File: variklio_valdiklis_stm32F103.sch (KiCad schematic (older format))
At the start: 88 parts, among them Q1 BC807, Q2 IRF830, Q3 IRF830, Q4 IRF830, Q5 IRF830, Q6 IRF830, Q7 IRF830, U1 CNY17-1, U10 IR2101, U2 CNY17-1, U3 CNY17-1, U4 LNK304G, U5 PC817, U6 SIP21106, U7 STM32F103C8Tx, U8 IR2101, U9 IR2101

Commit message: stm32f103c8tx schemos ir plokstes ruosimas
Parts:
- removed L2: 1mH/280mA, symbol Device:L
- added C1, C3, C4: 120x400V, Capacitor_THT:CP_Radial_D22.0mm_P10.00mm_SnapIn, symbol variklio_valdiklis_stm32F103-rescue:CP-Device
- added C14: 100n, Capacitor_SMD:C_0805_2012Metric, symbol variklio_valdiklis_stm32F103-rescue:C-Device
- added C24: 1n0, Capacitor_SMD:C_0805_2012Metric, symbol variklio_valdiklis_stm32F103-rescue:C-Device
- added D10, D20, D8, D9: LL4148, Diode_SMD:D_MiniMELF, symbol variklio_valdiklis_stm32F103-rescue:D-Device
- added D22, D23, D24, D25: D, Diode_THT:D_DO-201AD_P15.24mm_Horizontal, symbol variklio_valdiklis_stm32F103-rescue:D-Device
- added F1: 3A, Fuse:Fuseholder_TR5_Littelfuse_No560_No460, symbol Device:Fuse
- added F2: 5A, Fuse:Fuseholder_TR5_Littelfuse_No560_No460, symbol Device:Fuse
- added J1: Conn_01x05, valdiklio_footprints:Jungtis, symbol Connector_Generic:Conn_01x05
- added J3: ISP_SWD_Connector, mech:ISP_SWD_Connector, symbol mech:ISP_SWD_Connector
- added L2: 1mH/280mA, Inductor_THT:L_Radial_D7.8mm_P5.00mm_Fastron_07HCP, symbol Device:L_Core_Iron
- added R16: 100k, Resistor_SMD:R_0805_2012Metric, symbol variklio_valdiklis_stm32F103-rescue:R-Device
- added R18, R38, R39: 1K0, Resistor_SMD:R_0805_2012Metric, symbol variklio_valdiklis_stm32F103-rescue:R-Device
- added R19, R20, R21: 1k0, Resistor_SMD:R_0805_2012Metric, symbol variklio_valdiklis_stm32F103-rescue:R-Device
- added R34: 0R1, Resistor_THT:R_Axial_DIN0309_L9.0mm_D3.2mm_P12.70mm_Horizontal, symbol variklio_valdiklis_stm32F103-rescue:R_US-Device
- added R40: 220k, Resistor_THT:R_Axial_DIN0411_L9.9mm_D3.6mm_P12.70mm_Horizontal, symbol variklio_valdiklis_stm32F103-rescue:R-Device
- added RV1, RV2: Varistor, Varistor:RV_Disc_D9mm_W4mm_P5mm, symbol Device:Varistor
- added TH1: 33R, Varistor:RV_Disc_D9mm_W4mm_P5mm, symbol Device:Thermistor_PTC
- added TH2: 10K, symbol Device:Thermistor_NTC
- C10: renamed from C?; symbol Device:C -> variklio_valdiklis_stm32F103-rescue:C-Device
- C11: renamed from C7; symbol Device:C -> variklio_valdiklis_stm32F103-rescue:C-Device
- C12: renamed from C8; value 0.1 -> 100n; symbol Device:C -> variklio_valdiklis_stm32F103-rescue:C-Device
- C13: renamed from C9; footprint Capacitor_THT:C_Radial_D6.3mm_H5.0mm_P2.50mm -> Capacitor_THT:CP_Radial_D6.3mm_P2.50mm; symbol Device:CP -> variklio_valdiklis_stm32F103-rescue:CP-Device
- C15: renamed from C10; value C -> 100n; symbol Device:C -> variklio_valdiklis_stm32F103-rescue:C-Device
- C16: renamed from C11; value C -> 100n; symbol Device:C -> variklio_valdiklis_stm32F103-rescue:C-Device
- C17: renamed from C12; value C -> 100n; symbol Device:C -> variklio_valdiklis_stm32F103-rescue:C-Device
- C18: renamed from C13; symbol Device:C -> variklio_valdiklis_stm32F103-rescue:C-Device
- C19: renamed from C14; symbol Device:C -> variklio_valdiklis_stm32F103-rescue:C-Device
- C2: renamed from C1; footprint Capacitor_THT:C_Radial_D10.0mm_H20.0mm_P5.00mm -> Capacitor_THT:CP_Radial_D10.0mm_P5.00mm; symbol Device:CP -> variklio_valdiklis_stm32F103-rescue:CP-Device
- C20: renamed from C15; symbol Device:C -> variklio_valdiklis_stm32F103-rescue:C-Device
- C21: renamed from C16; symbol Device:C -> variklio_valdiklis_stm32F103-rescue:C-Device
- C22: renamed from C17; symbol Device:C -> variklio_valdiklis_stm32F103-rescue:C-Device
- C23: renamed from C18; symbol Device:C -> variklio_valdiklis_stm32F103-rescue:C-Device
- C5: renamed from C2; footprint Capacitor_THT:C_Radial_D10.0mm_H20.0mm_P5.00mm -> Capacitor_THT:CP_Radial_D10.0mm_P5.00mm; symbol Device:CP -> variklio_valdiklis_stm32F103-rescue:CP-Device
- C6: renamed from C5; symbol Device:CP -> variklio_valdiklis_stm32F103-rescue:CP-Device
- C7: renamed from C3; symbol Device:C -> variklio_valdiklis_stm32F103-rescue:C-Device
- C8: renamed from C4; footprint Capacitor_THT:C_Radial_D6.3mm_H5.0mm_P2.50mm -> Capacitor_THT:CP_Radial_D6.3mm_P2.50mm; symbol Device:CP -> variklio_valdiklis_stm32F103-rescue:CP-Device
- C9: renamed from C6; symbol Device:C -> variklio_valdiklis_stm32F103-rescue:C-Device
- D11: renamed from D6; value US1J -> UF4005; footprint (none) -> Diode_THT:D_DO-41_SOD81_P7.62mm_Horizontal; symbol Device:D -> variklio_valdiklis_stm32F103-rescue:D-Device
- D12: renamed from D7; value US1J -> UF4005; footprint (none) -> Diode_THT:D_DO-41_SOD81_P7.62mm_Horizontal; symbol Device:D -> variklio_valdiklis_stm32F103-rescue:D-Device
- D13: renamed from D8; value US1J -> UF4005; footprint (none) -> Diode_THT:D_DO-41_SOD81_P7.62mm_Horizontal; symbol Device:D -> variklio_valdiklis_stm32F103-rescue:D-Device
- D14: renamed from D9; footprint (none) -> Diode_SMD:D_MiniMELF; symbol Device:D -> variklio_valdiklis_stm32F103-rescue:D-Device
- D15: renamed from D10; footprint (none) -> Diode_SMD:D_MiniMELF; symbol Device:D -> variklio_valdiklis_stm32F103-rescue:D-Device
- D16: renamed from D11; footprint (none) -> Diode_SMD:D_MiniMELF; symbol Device:D -> variklio_valdiklis_stm32F103-rescue:D-Device
- D17: renamed from D12; footprint (none) -> Diode_SMD:D_MiniMELF; symbol Device:D -> variklio_valdiklis_stm32F103-rescue:D-Device
- D18: renamed from D13; footprint (none) -> Diode_SMD:D_MiniMELF; symbol Device:D -> variklio_valdiklis_stm32F103-rescue:D-Device
- D19: renamed from D14; footprint (none) -> Diode_SMD:D_MiniMELF; symbol Device:D -> variklio_valdiklis_stm32F103-rescue:D-Device
- D2: renamed from D1; symbol Device:D -> variklio_valdiklis_stm32F103-rescue:D-Device
- D3: renamed from D2; symbol Device:D -> variklio_valdiklis_stm32F103-rescue:D-Device
- D4: renamed from D3; value LL4005 -> LL4148; footprint Diode_SMD:D_MELF -> Diode_SMD:D_MiniMELF; symbol Device:D -> variklio_valdiklis_stm32F103-rescue:D-Device
- D5: renamed from D4; footprint (none) -> Diode_THT:D_DO-41_SOD81_P10.16mm_Horizontal; symbol Device:D -> variklio_valdiklis_stm32F103-rescue:D-Device
- D6: renamed from D5; value D_Zener -> 12V; footprint (none) -> Diode_SMD:D_MiniMELF; symbol Device:D_Zener -> variklio_valdiklis_stm32F103-rescue:D_Zener-Device
- D7: renamed from D?; value LL4005 -> LL4148; footprint Diode_SMD:D_MELF -> Diode_SMD:D_MiniMELF; symbol Device:D -> variklio_valdiklis_stm32F103-rescue:D-Device
- L1: footprint (none) -> Inductor_SMD:L_Vishay_IHSM-3825; symbol Device:L -> variklio_valdiklis_stm32F103-rescue:L-Device
- Q1: symbol Transistor_BJT:BC807 -> variklio_valdiklis_stm32F103-rescue:BC807-Transistor_BJT
- Q2, Q3, Q4, Q5, Q6, Q7: symbol Transistor_FET:IRF740 -> variklio_valdiklis_stm32F103-rescue:IRF740-Transistor_FET
- R1: renamed from R2; symbol Device:R -> variklio_valdiklis_stm32F103-rescue:R-Device
- R10, R11, R12, R13, R14, R15, R5, R6: symbol Device:R -> variklio_valdiklis_stm32F103-rescue:R-Device
- R17: renamed from R?; symbol Device:R -> variklio_valdiklis_stm32F103-rescue:R-Device
- R2: renamed from R3; symbol Device:R -> variklio_valdiklis_stm32F103-rescue:R-Device
- R22: renamed from R16; value R -> 47R; symbol Device:R -> variklio_valdiklis_stm32F103-rescue:R-Device
- R23: renamed from R17; value R -> 47R; symbol Device:R -> variklio_valdiklis_stm32F103-rescue:R-Device
- R24: renamed from R18; value R -> 47R; symbol Device:R -> variklio_valdiklis_stm32F103-rescue:R-Device
- R25: renamed from R19; value R -> 47R; symbol Device:R -> variklio_valdiklis_stm32F103-rescue:R-Device
- R26: renamed from R20; value R -> 47R; symbol Device:R -> variklio_valdiklis_stm32F103-rescue:R-Device
- R27: renamed from R21; value R -> 47R; symbol Device:R -> variklio_valdiklis_stm32F103-rescue:R-Device
- R28: renamed from R22; symbol Device:R -> variklio_valdiklis_stm32F103-rescue:R-Device
- R29: renamed from R23; symbol Device:R -> variklio_valdiklis_stm32F103-rescue:R-Device
- R3: renamed from R4; symbol Device:R -> variklio_valdiklis_stm32F103-rescue:R-Device
- R30: renamed from R24; symbol Device:R -> variklio_valdiklis_stm32F103-rescue:R-Device
- R31: renamed from R25; symbol Device:R -> variklio_valdiklis_stm32F103-rescue:R-Device
- R32: renamed from R26; symbol Device:R -> variklio_valdiklis_stm32F103-rescue:R-Device
- R33: renamed from R27; symbol Device:R -> variklio_valdiklis_stm32F103-rescue:R-Device
- R35: renamed from R28; symbol Device:R_US -> variklio_valdiklis_stm32F103-rescue:R_US-Device
- R36: renamed from R29; symbol Device:R_US -> variklio_valdiklis_stm32F103-rescue:R_US-Device
- R37: renamed from R30; symbol Device:R_US -> variklio_valdiklis_stm32F103-rescue:R_US-Device
- R4: renamed from R1; footprint (none) -> Resistor_THT:R_Axial_DIN0411_L9.9mm_D3.6mm_P12.70mm_Horizontal; symbol Device:R -> variklio_valdiklis_stm32F103-rescue:R-Device
- R7: renamed from R8; symbol Device:R -> variklio_valdiklis_stm32F103-rescue:R-Device
- R8: renamed from R9; symbol Device:R -> variklio_valdiklis_stm32F103-rescue:R-Device
- R9: renamed from R7; symbol Device:R -> variklio_valdiklis_stm32F103-rescue:R-Device
- U1, U2, U3: symbol Isolator:CNY17-1 -> variklio_valdiklis_stm32F103-rescue:CNY17-1-Isolator
- U10, U8, U9: footprint (none) -> Package_SO:SOIC-8_3.9x4.9mm_P1.27mm; symbol Driver_FET:IR2101 -> variklio_valdiklis_stm32F103-rescue:IR2101-Driver_FET
- U4: symbol Regulator_Switching:LNK304G -> variklio_valdiklis_stm32F103-rescue:LNK304G-Regulator_Switching
- U5: footprint Package_DIP:DIP-4_W7.62mm -> Package_DIP:DIP-4_W10.16mm_LongPads; symbol Isolator:PC817 -> variklio_valdiklis_stm32F103-rescue:PC817-Isolator
- U6: footprint TO_SOT_Packages_SMD:SOT-23-5 -> Package_TO_SOT_SMD:SOT-23-5; symbol disc:USTAB_SIP21106-DT-33 -> variklio_valdiklis_stm32F103-rescue:USTAB_SIP21106-DT-33-disc
- VP1: symbol Device:R_POT_TRIM -> variklio_valdiklis_stm32F103-rescue:R_POT_TRIM-Device
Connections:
- net labels added: VB, ~NRST
- net labels removed: ~SA, ~SB, ~SC
- wire segments 350 -> 423
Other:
- moved on the sheet: C11, C12, C13, C15, C16, C17, C18, C19, C2, C20, C21, C22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

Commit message: 2019.10.10
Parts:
- J3: symbol mech:ISP_SWD_Connector -> variklio_valdiklis_stm32F103-rescue:ISP_SWD_Connector-mech
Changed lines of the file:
@@
 EESchema Schematic File Version 4
 LIBS:variklio_valdiklis_stm32F103-cache
-EELAYER 30 0
+EELAYER 29 0
 EELAYER END
 $Descr A3 16535 11693
@@
 	7950 3050 8500 3050
 $Comp
-L mech:ISP_SWD_Connector J3
+L variklio_valdiklis_stm32F103-rescue:ISP_SWD_Connector-mech J3
 U 1 1 5DDC24FE
 P 7950 2650

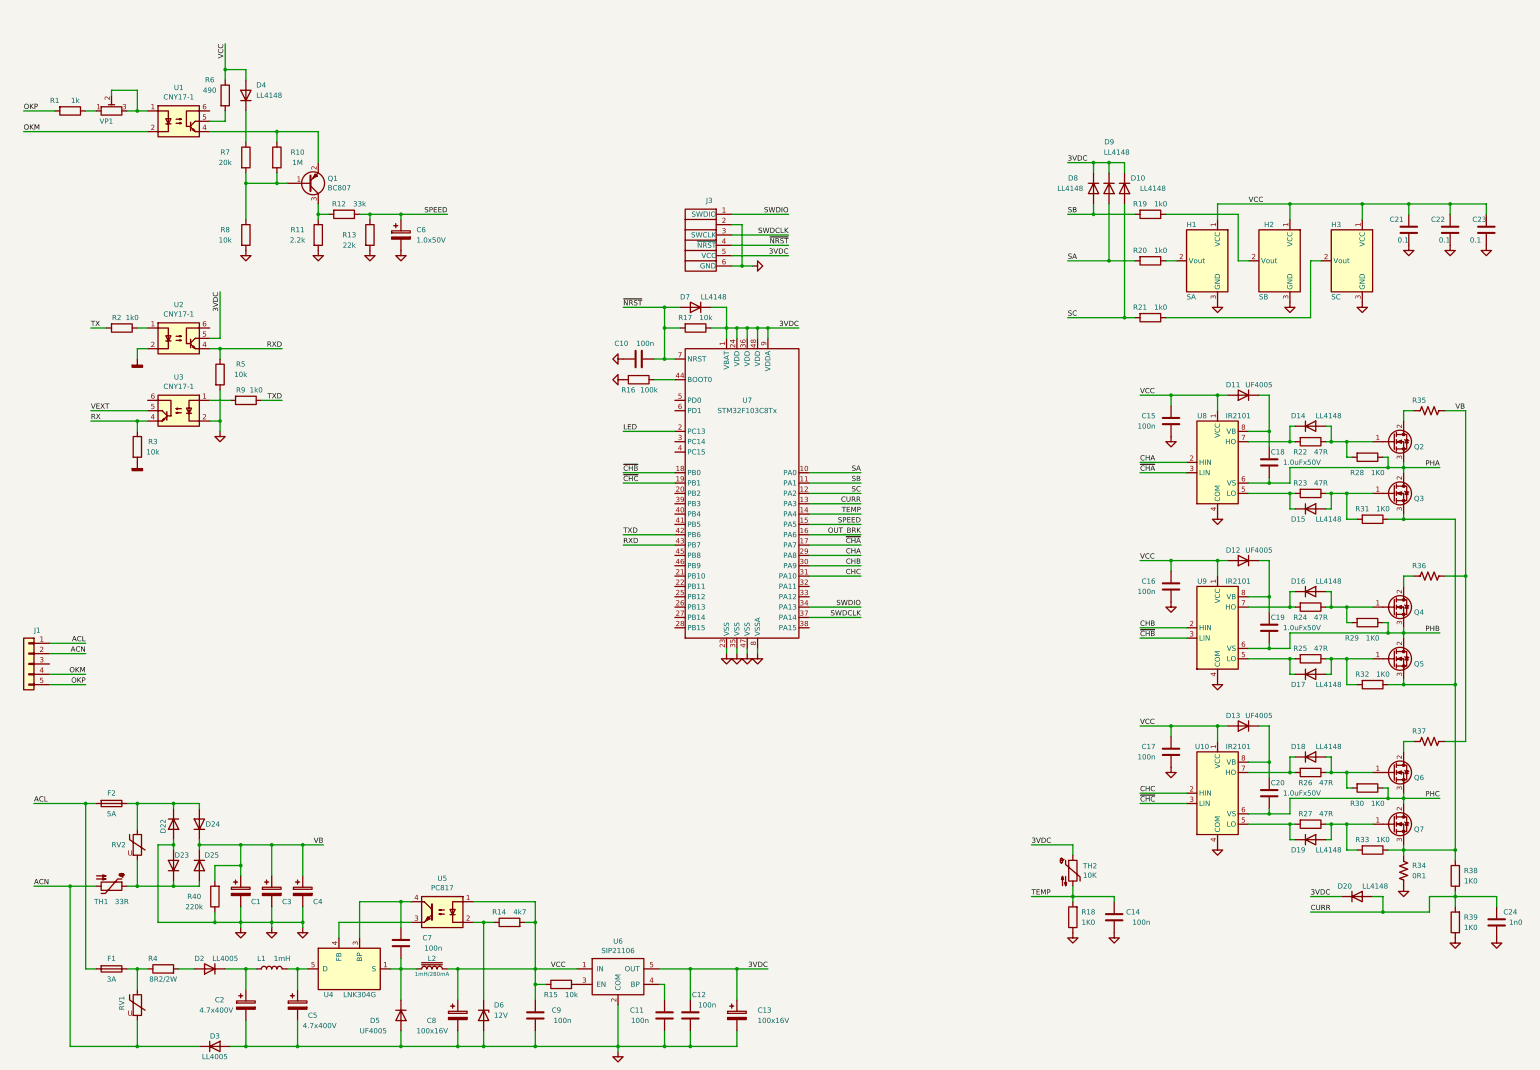
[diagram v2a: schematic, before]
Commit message: plokstes testavimams
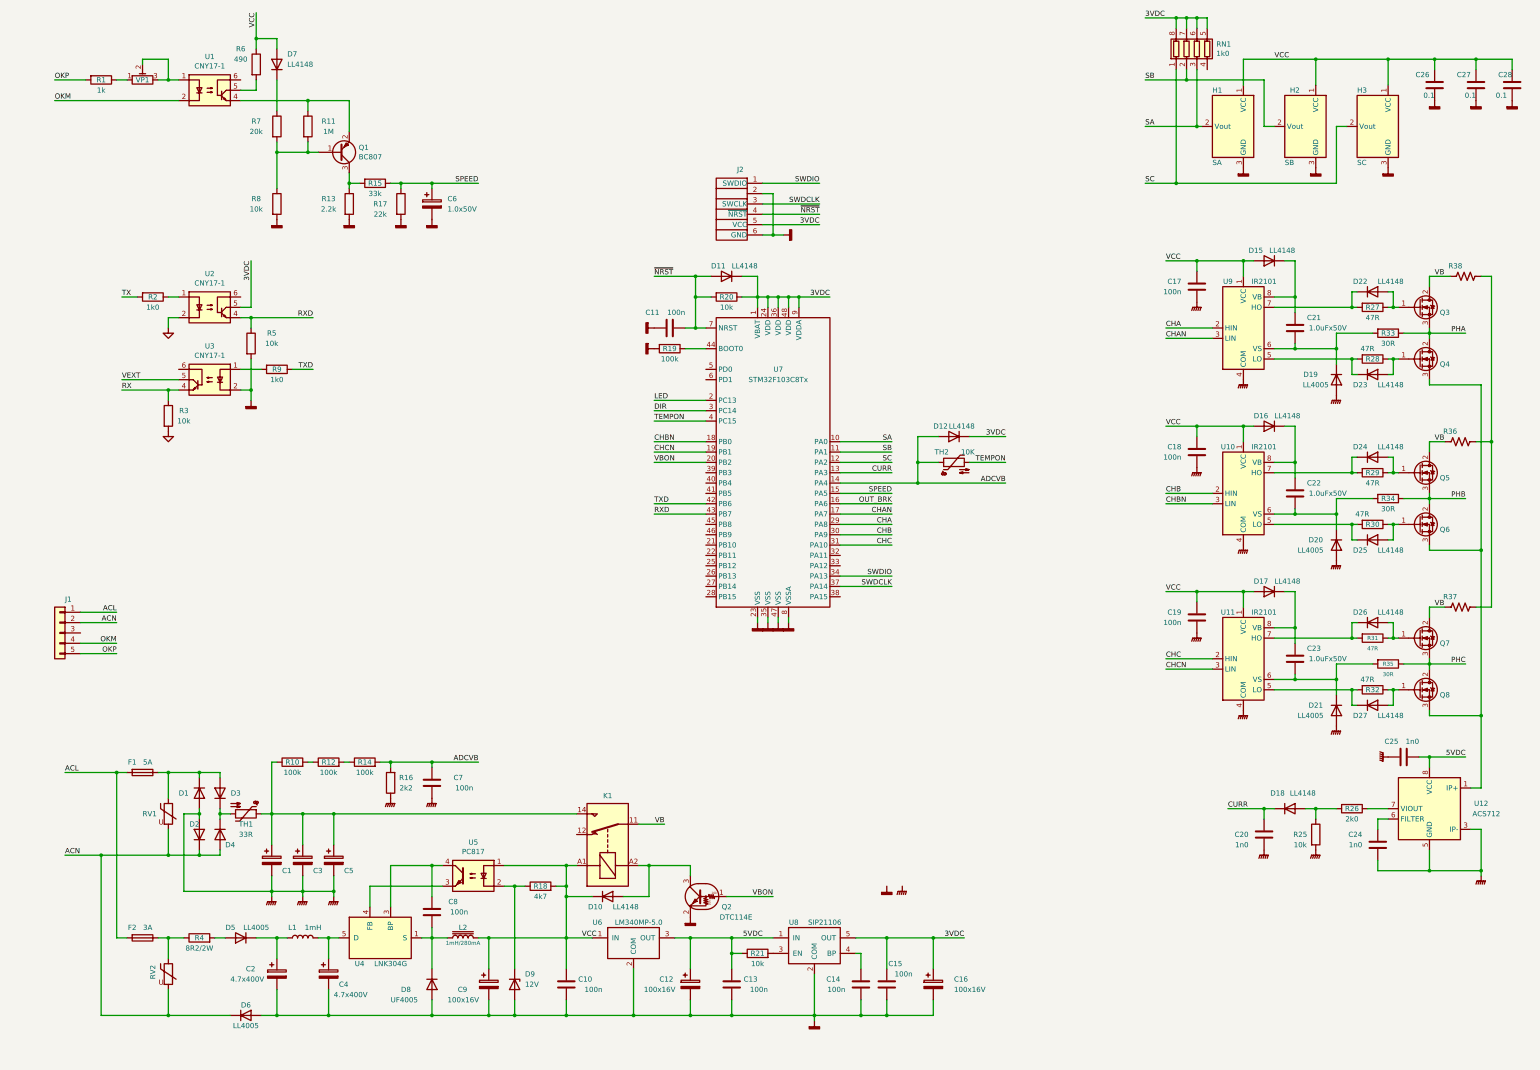
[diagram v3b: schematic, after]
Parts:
- removed C14: 100n, Capacitor_SMD:C_0805_2012Metric, symbol variklio_valdiklis_stm32F103-rescue:C-Device
- removed D20, D8, D9: LL4148, Diode_SMD:D_MiniMELF, symbol variklio_valdiklis_stm32F103-rescue:D-Device
- removed R18, R28, R29, R30, R31, R32, R39: 1K0, Resistor_SMD:R_0805_2012Metric, symbol variklio_valdiklis_stm32F103-rescue:R-Device
- removed R19, R20, R21: 1k0, Resistor_SMD:R_0805_2012Metric, symbol variklio_valdiklis_stm32F103-rescue:R-Device
- removed R34: 0R1, Resistor_THT:R_Axial_DIN0309_L9.0mm_D3.2mm_P12.70mm_Horizontal, symbol variklio_valdiklis_stm32F103-rescue:R_US-Device
- removed R40: 220k, Resistor_THT:R_Axial_DIN0411_L9.9mm_D3.6mm_P12.70mm_Horizontal, symbol variklio_valdiklis_stm32F103-rescue:R-Device
- added C12: 100x16V, Capacitor_THT:CP_Radial_D6.3mm_P2.50mm, symbol variklio_valdiklis_stm32F103-rescue:CP-Device
- added C13, C7: 100n, Capacitor_SMD:C_0805_2012Metric, symbol variklio_valdiklis_stm32F103-rescue:C-Device
- added C20, C25: 1n0, Capacitor_SMD:C_0805_2012Metric, symbol variklio_valdiklis_stm32F103-rescue:C-Device
- added D12, D15, D16, D17, D18: LL4148, Diode_SMD:D_MiniMELF, symbol variklio_valdiklis_stm32F103-rescue:D-Device
- added K1: Omron, Relay_THT:Relay_SPDT_Finder_34.51_Vertical, symbol Relay:FINDER-32.21-x000
- added Q2: DTC114E, Package_TO_SOT_SMD:SOT-23, symbol Transistor_BJT:DTC114E
- added R10, R12, R14: 100k, Resistor_SMD:R_1206_3216Metric, symbol variklio_valdiklis_stm32F103-rescue:R-Device
- added R16: 2k2, Resistor_SMD:R_0805_2012Metric, symbol variklio_valdiklis_stm32F103-rescue:R-Device
- added R25: 10k, Resistor_SMD:R_0805_2012Metric, symbol variklio_valdiklis_stm32F103-rescue:R-Device
- added R34, R35: 30R, Resistor_SMD:R_0805_2012Metric, symbol variklio_valdiklis_stm32F103-rescue:R-Device
- added RN1: 1k0, Resistor_SMD:R_Array_Convex_4x0603, symbol Device:R_Pack04
- added U12: ACS712, Package_SO:SOIC-8_3.9x4.9mm_P1.27mm, symbol Sensor_Current:ACS712xLCTR-05B
- added U6: LM340MP-5.0, disc:LM340_SOT-223, symbol disc:LM340MP-5.0
- D19: renamed from D11; value UF4005 -> LL4005; footprint Diode_THT:D_DO-41_SOD81_P7.62mm_Horizontal -> Diode_SMD:D_MELF
- D20: renamed from D12; value UF4005 -> LL4005; footprint Diode_THT:D_DO-41_SOD81_P7.62mm_Horizontal -> Diode_SMD:D_MELF
- D21: renamed from D13; value UF4005 -> LL4005; footprint Diode_THT:D_DO-41_SOD81_P7.62mm_Horizontal -> Diode_SMD:D_MELF
- R26: renamed from R38; value 1K0 -> 2k0
- R33: value 1K0 -> 30R
- renumbered C9 to C10, C10 to C11, C11 to C14, C12 to C15, C13 to C16, C15 to C17, C16 to C18, C17 to C19, C18 to C21, C19 to C22, C20 to C23, C21 to C26, C22 to C27, C23 to C28, C5 to C4, C4 to C5, C7 to C8, C8 to C9, D22 to D1, D7 to D11, D23 to D2, D14 to D22, D15 to D23, D16 to D24, D17 to D25, D18 to D26, D19 to D27, D24 to D3, D25 to D4, D2 to D5, D3 to D6, D4 to D7, D5 to D8, D6 to D9, F2 to F1, F1 to F2, J3 to J2, Q2 to Q3, Q3 to Q4, Q4 to Q5, Q5 to Q6, Q6 to Q7, Q7 to Q8, R10 to R11, R11 to R13, R12 to R15, R13 to R17, R14 to R18, R16 to R19, R17 to R20, R15 to R21, R22 to R27, R23 to R28, R24 to R29, R25 to R30, R26 to R31, R27 to R32, R35 to R38, RV2 to RV1, RV1 to RV2, U9 to U10, U10 to U11, U6 to U8, U8 to U9
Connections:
- net 3VDC: now also D12.1 (K), RN1.5 (R4.2), RN1.6 (R3.2), RN1.7 (R2.2), RN1.8 (R1.2); no longer D10.1 (K), TH2.1
- net ACN: now also D2.1 (K), D4.2 (A), RV1.2; no longer TH1.2
- net CURR: now also C20.2, D18.1 (K); no longer C24.2, R26.1
- net GND: now also R3.2, U2.2; no longer C1.2, C10.1, C11.1, C14.1, C15.1, C16.2, C17.1, C18.1, C19.1, C2.2, C24.1, C26.1, C27.1, C28.1, C3.2, C4.2, C5.2, C6.2, C9.2, D1.2 (A), D2.2 (A), D6.2 (A), D8.2 (A), D9.2 (A), H1.3 (GND), H2.3 (GND), H3.3 (GND), J2.2, J2.6 (GND), R13.2, R17.2, R19.2, R5.2, R8.2, U10.4 (COM), U11.4 (COM), U3.2, U7.23 (VSS), U7.35 (VSS), U7.47 (VSS), U7.8 (VSSA), U8.2 (COM), U9.4 (COM)
- net GNDD: now also C10.1, C11.1, C14.1, C15.1, C16.2, C2.2, C26.1, C27.1, C28.1, C4.2, C6.2, C9.2, D6.2 (A), D8.2 (A), D9.2 (A), H1.3 (GND), H2.3 (GND), H3.3 (GND), J2.2, J2.6 (GND), R13.2, R17.2, R19.2, R5.2, R8.2, U3.2, U7.23 (VSS), U7.35 (VSS), U7.47 (VSS), U7.8 (VSSA), U8.2 (COM), C12.2, C13.1, Q2.2 (E), U6.2 (COM); no longer R3.2, U2.2
- net PHA: now also R33.1; no longer C21.1, U9.6 (VS)
- net PHB: now also R34.1; no longer C22.1, U10.6 (VS)
- net PHC: now also R35.1; no longer C23.1, U11.6 (VS)
- net SA: now also H1.2 (Vout), RN1.3 (R3.1)
- net SB: now also H2.2 (Vout), RN1.2 (R2.1)
- net SC: now also H3.2 (Vout), RN1.1 (R1.1); no longer D10.2 (A)
- net VB: now also Q3.2 (D), Q5.2 (D), Q7.2 (D), R36.2, R37.2, R38.2, K1.11; no longer C1.1, C3.1, C5.1, D3.1 (K), D4.1 (K), R36.1, R37.1, R38.1
- net VCC: now also D10.1 (K), D15.2 (A), D16.2 (A), D17.2 (A), K1.A1, U6.1 (IN); no longer D19.2 (A), D20.2 (A), D21.2 (A), R21.1, U8.1 (IN)
- net at Q4.3 (S), Q6.3 (S), Q8.3 (S): now also U12.1 (IP+), U12.2 (IP+); no longer R26.2, R33.1
- net at C21.2, U9.8 (VB): now also D15.1 (K); no longer D19.1 (K)
- net VBON: now reaches U7.20 (PB2)
- net VBON: now also Q2.1 (B)
- net DIR: now reaches U7.3 (PC14)
- net TEMPON: now reaches U7.4 (PC15)
- net TEMPON: now also TH2.2
- net at C22.2, U10.8 (VB): now also D16.1 (K); no longer D20.1 (K)
- net at C23.2, U11.8 (VB): now also D17.1 (K); no longer D21.1 (K)
- net at D27.2 (A), Q8.1 (G), R32.1: no longer R33.2
- net TEMP renamed ADCVB
- net ADCVB: now also TH2.1, C7.2, D12.2 (A), R14.2, R16.2; no longer TH2.2
- net ~CHA renamed CHAN
- net ~CHB renamed CHBN
- net ~CHC renamed CHCN
- new net: R26.1, U12.7 (VIOUT)
- new net: D18.2 (A), R25.1, R26.2
- new net: C21.1, D19.1 (K), R33.2, U9.6 (VS)
- new net: C24.2, U12.6 (FILTER)
- new net: C22.1, D20.1 (K), R34.2, U10.6 (VS)
- new net: C23.1, D21.1 (K), R35.2, U11.6 (VS)
- new net: C1.1, C3.1, C5.1, K1.14, R10.1, TH1.1
- new net: D3.1 (K), D4.1 (K), TH1.2
- new net: R36.1, R37.1, R38.1
- new net: D10.2 (A), K1.A2, Q2.3 (C)
- new net: R10.2, R12.1
- new net: R12.2, R14.1
- new net 5VDC: C12.1, C13.2, C25.2, R21.1, U12.8 (VCC), U6.3 (OUT), U8.1 (IN)
- new net GNDPWR: C1.2, C17.1, C18.1, C19.1, C20.1, C24.1, C25.1, C3.2, C5.2, C7.1, D1.2 (A), D19.2 (A), D2.2 (A), D20.2 (A), D21.2 (A), R16.1, R25.2, U10.4 (COM), U11.4 (COM), U12.3 (IP-), U12.4 (IP-), U12.5 (GND), U9.4 (COM)
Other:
- moved on the sheet: C1, C10, C11, C14, C15, C16, C17, C18, C19, C2, C21, C22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
